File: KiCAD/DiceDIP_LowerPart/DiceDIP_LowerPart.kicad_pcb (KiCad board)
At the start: 2 copper layers, 40 x 40 mm, 21 parts, among them J1 Conn_01x03, J4 Conn_01x06, Q1 BC547, U1 4029, U2 4093

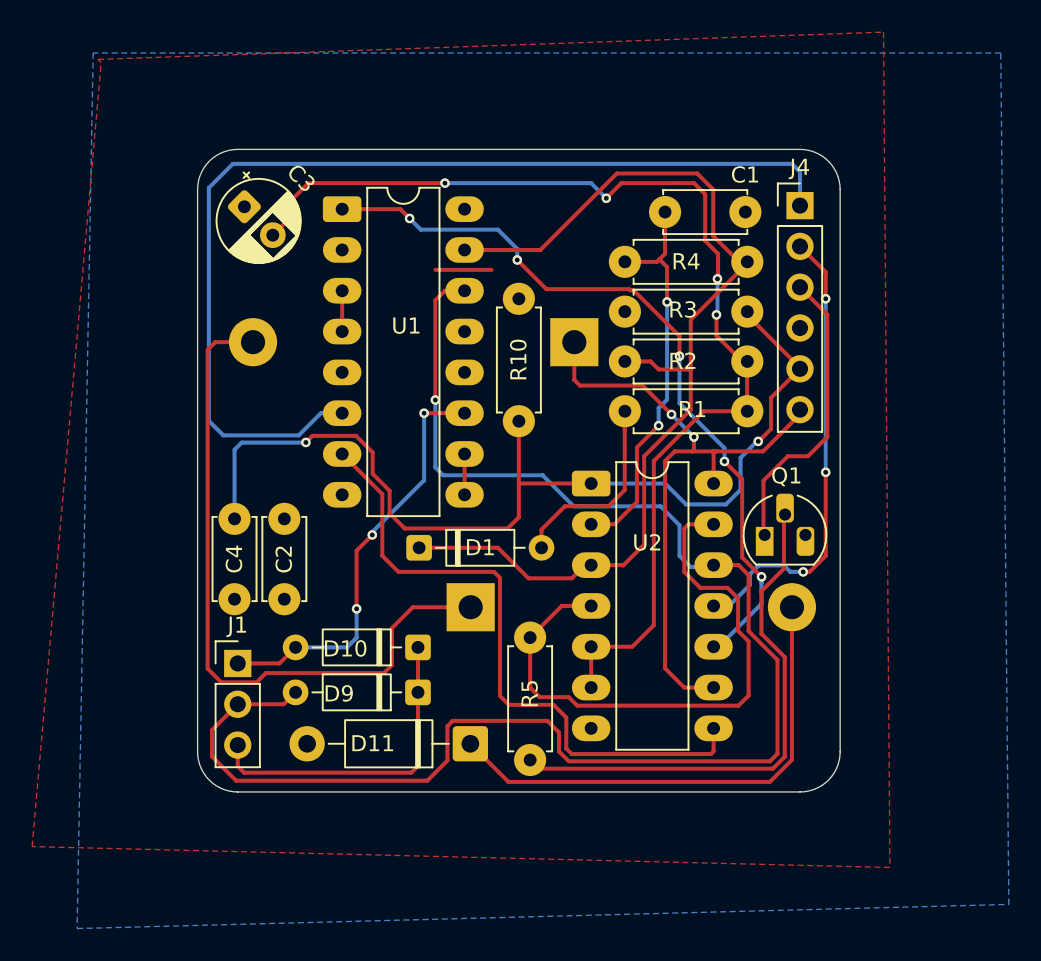
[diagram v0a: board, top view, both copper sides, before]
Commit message: minor changes
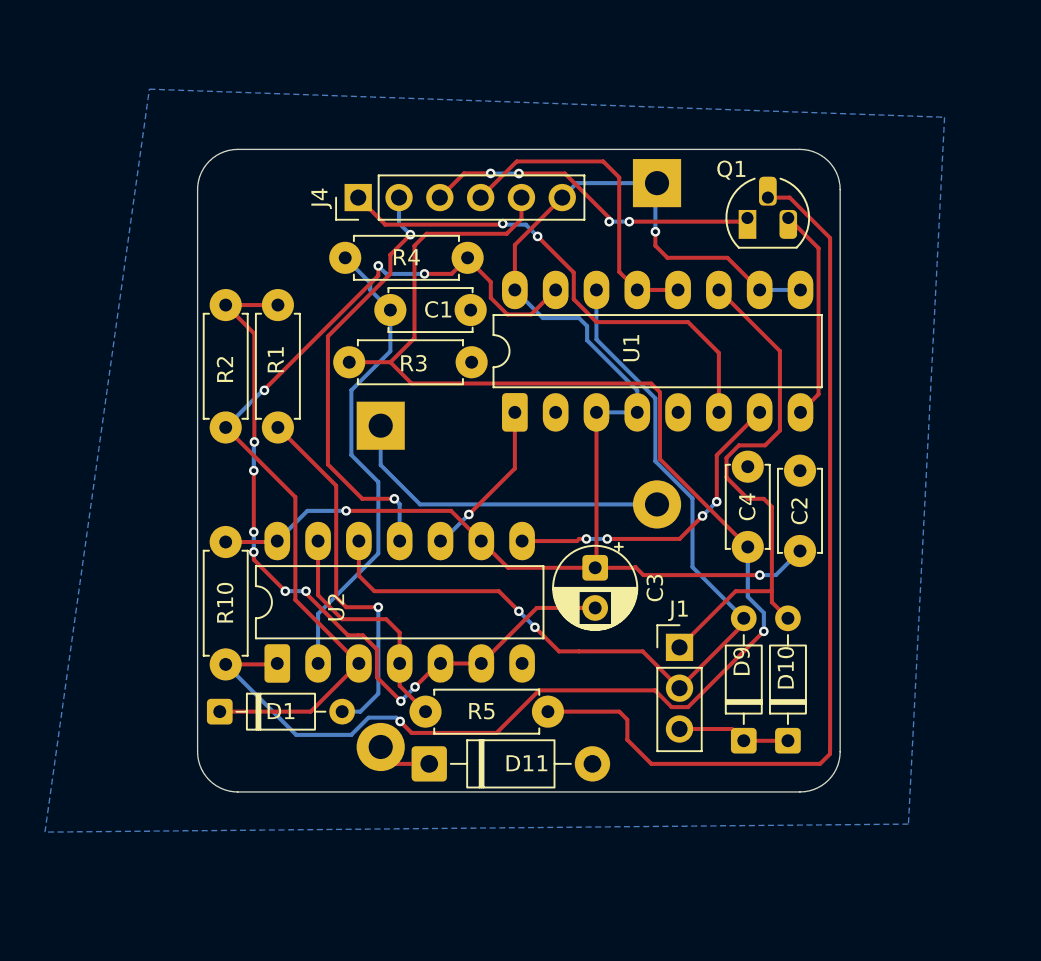
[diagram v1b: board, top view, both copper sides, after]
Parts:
- moved C2 33.1 mm to (137.5, 95.0), turned to -90 degrees
- moved C4 33.0 mm to (134.2, 94.8), turned to -90 degrees
- moved C3 31.3 mm to (124.8, 101.0), turned to -90 degrees
- moved J1 27.5 mm to (130.0, 106.0)
- moved J4 27.5 mm to (110.0, 78.0), turned to 90 degrees
- moved R2 25.2 mm to (101.8, 92.3), turned to 90 degrees
- moved D10 23.8 mm to (136.8, 111.8), turned to 90 degrees
- moved R10 23.7 mm to (101.8, 107.1)
- moved U2 22.5 mm to (105.0, 107.0), turned to 90 degrees
- moved R1 21.6 mm to (105.0, 92.3), turned to 90 degrees
- moved D9 20.5 mm to (134.0, 111.8), turned to 90 degrees
- moved Q1 19.8 mm to (134.2, 79.3)
- moved C1 18.2 mm to (117.0, 85.0)
- moved R4 17.4 mm to (109.2, 81.8)
- moved U1 16.6 mm to (119.8, 91.4), turned to 90 degrees
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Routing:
- net Net-(D9-A): track 97.4 -> 55.3 mm, vias 1 -> 2
- net VCC: track 50.8 -> 90.8 mm, vias 2 -> 3
- net Net-(U1-PE): track 47.6 -> 9.99 mm, vias 5 -> 1
- net SW_V2: track 61.2 -> 97.1 mm
- net SW_V1: track 0.00 -> 33.6 mm
- net Net-(J4-Pin_1): track 63.5 -> 31.2 mm, vias 0 -> 2
- net Net-(BT1--): track 31.1 -> 3.45 mm
- net Net-(Q1-B): track 32.7 -> 56.9 mm
- net Net-(BT1-+): track 42.9 -> 20.7 mm
- net Net-(R5-Pad1): track 37.0 -> 15.0 mm
- net Net-(C3-Pad2): track 69.4 -> 48.2 mm, vias 4 -> 8
- net Net-(U1-Cout): track 40.1 -> 19.8 mm, vias 0 -> 4
- net Net-(D10-K): track 20.3 -> 7.05 mm
- net Net-(D1-A): track 12.9 -> 23.0 mm, vias 0 -> 1
- net Net-(D10-A): track 26.7 -> 33.7 mm, vias 3 -> 0
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- removed copper zone on F.Cu, net VCC
